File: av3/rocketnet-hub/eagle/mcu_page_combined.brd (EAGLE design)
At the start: 112.7 x 76.3 mm, 393 parts, among them J1 ROCKETNET-CONNECTOR-16M, J10 ROCKETNET-UMBILICAL-12, J11 1.27MM_HDR_2X5, J12 1.27MM_HDR_2X12X1, J2 ROCKETNET-CONNECTOR-16M, J3 ROCKETNET-CONNECTOR-16M, J4 ROCKETNET-CONNECTOR-16M, J5 1.27MM_HDR_2X12X1, J6 ROCKETNET-CONNECTOR-16M, J7 ROCKETNET-CONNECTOR-16M, J8 ROCKETNET-CONNECTOR-16M, J9 ROCKETNET-BATTERY-14, Q1 25MHz, Q2 FDS6680ASOIC-8, Q3 FDS6680ASOIC-8, Q4 FDS6680ASOIC-8, Q5 SIS412DNSOP-8, Q6 BSS138W-7-F, Q7 SIS412DNSOP-8, U1 STM32F407V100-PIN_QFP, U2 BQ24725QFN-20

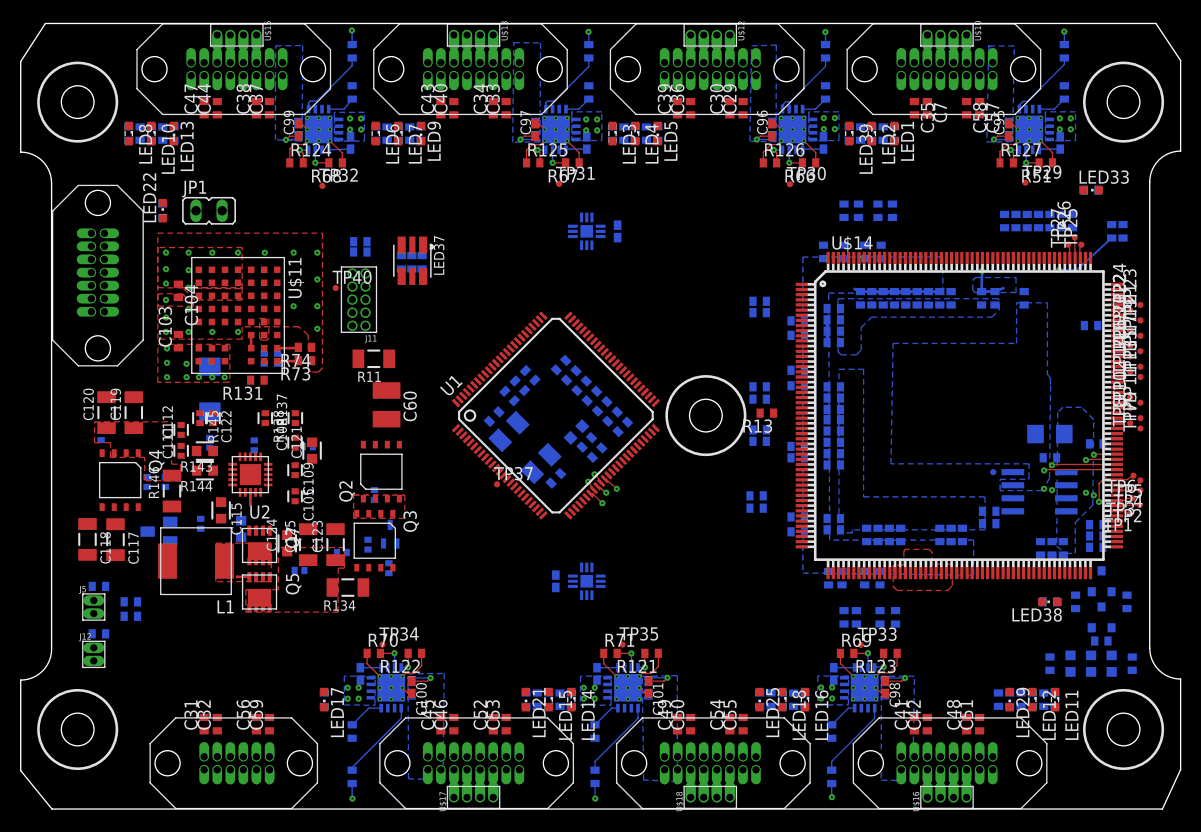
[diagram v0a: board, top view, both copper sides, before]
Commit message: Fixed ground vias DRC errors
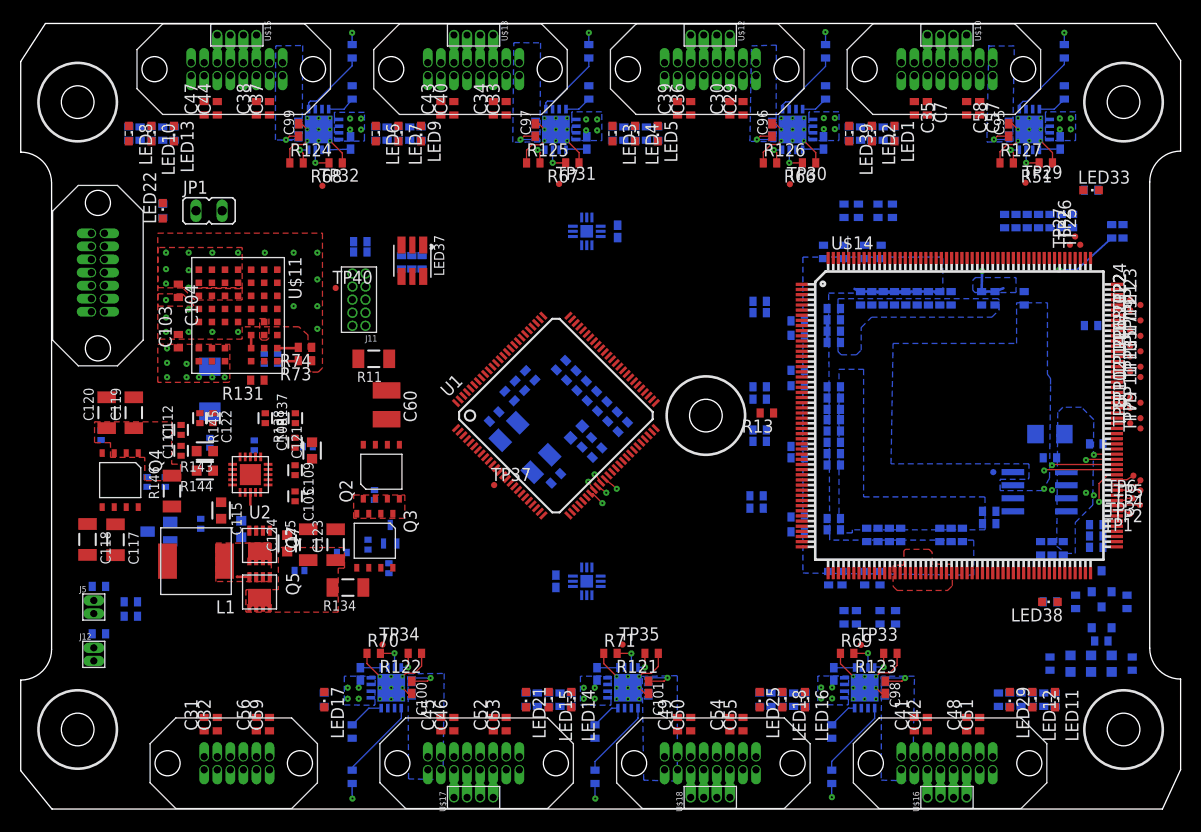
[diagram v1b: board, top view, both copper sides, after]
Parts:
- moved TP37 0.30 mm to (46.0, 31.4)
- moved TP27 0.19 mm to (102.0, 54.7)
- moved TP25 0.11 mm to (103.0, 54.7)
- moved TP26 0.10 mm to (102.5, 55.5)
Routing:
- net N$95: track 2.01 -> 0.00 mm
- net N$93: track 1.38 -> 0.00 mm
- net N$97: track 1.37 -> 0.00 mm
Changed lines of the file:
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@@
 <layers>
 <layer number="1" name="Top" color="4" fill="1" visible="yes" active="yes"/>
-<layer number="2" name="GND" color="1" fill="3" visible="no" active="yes"/>
+<layer number="2" name="GND" color="1" fill="3" visible="yes" active="yes"/>
 <layer number="3" name="Power" color="4" fill="3" visible="no" active="yes"/>
 <layer number="14" name="NS" color="1" fill="6" visible="yes" active="yes"/>
@@
 <attribute name="TP_SIGNAL_NAME" value="" x="107.8" y="49.35" size="1.778" layer="27" rot="R90" display="off"/>
 </element>
-<element name="TP25" library="testpad" package="TP06R" value="TPTP06R" x="103.063" y="54.7096" rot="R90">
-<attribute name="TP_SIGNAL_NAME" value="" x="103.063" y="54.7096" size="1.778" layer="27" rot="R90" display="off"/>
+<element name="TP25" library="testpad" package="TP06R" value="TPTP06R" x="102.95" y="54.7" rot="R90">
+<attribute name="TP_SIGNAL_NAME" value="" x="102.95" y="54.7" size="1.778" layer="27" rot="R90" display="off"/>
 </element>
-<element name="TP26" library="testpad" package="TP06R" value="TPTP06R" x="102.413" y="55.4096" rot="R90">
-<attribute name="TP_SIGNAL_NAME" value="" x="102.413" y="55.4096" size="1.778" layer="27" rot="R90" display="off"/>
+<element name="TP26" library="testpad" package="TP06R" value="TPTP06R" x="102.45" y="55.5" rot="R90">
+<attribute name="TP_SIGNAL_NAME" value="" x="102.45" y="55.5" size="1.778" layer="27" rot="R90" display="off"/>
 </element>
-<element name="TP27" library="testpad" package="TP06R" value="TPTP06R" x="101.763" y="54.7096" rot="R90">
-<attribute name="TP_SIGNAL_NAME" value="" x="101.763" y="54.7096" size="1.778" layer="27" rot="R90" display="off"/>
+<element name="TP27" library="testpad" package="TP06R" value="TPTP06R" x="101.95" y="54.7" rot="R90">
+<attribute name="TP_SIGNAL_NAME" value="" x="101.95" y="54.7" size="1.778" layer="27" rot="R90" display="off"/>
 </element>
 <element name="R2" library="rcl" package="R0402" value="10" x="106" y="56" rot="MR90"/>
@@
 </element>
 <element name="D3" library="diode-0603" package="0603-B-NOSILK-DIODE" value="DIODE-0603" x="104" y="14" rot="MR90"/>
-<element name="TP37" library="testpad" package="TP06R" value="TPTP06R" x="46.2876" y="31.4218">
-<attribute name="TP_SIGNAL_NAME" value="" x="46.0876" y="31.4218" size="1.778" layer="27" display="off"/>
+<element name="TP37" library="testpad" package="TP06R" value="TPTP06R" x="46" y="31.35">
+<attribute name="TP_SIGNAL_NAME" value="" x="45.8" y="31.35" size="1.778" layer="27" display="off"/>
 </element>
 <element name="JP1" library="jumper" package="JP1" value="" x="18.3" y="58" rot="R270"/>
@@
 <wire x1="52.04038125" y1="42.540378125" x2="53.923328125" y2="47.094396875" width="0" layer="19" extent="1-16"/>
 </signal>
-<signal name="GND" class="1" airwireshidden="yes">
+<signal name="GND" class="1">
 <contactref element="U1" pad="10"/>
 <contactref element="C1" pad="2"/>
@@
 <wire x1="27" y1="66.45" x2="27.295" y2="66.448" width="0.127" layer="1"/>
 <wire x1="27.295" y1="66.448" x2="27.85" y2="65.9" width="0.127" layer="1"/>
-<wire x1="32.2" y1="74.15" x2="32.2" y2="75.5142" width="0.127" layer="16"/>
-<wire x1="32.2" y1="75.5142" x2="32.1818" y2="75.5142" width="0.127" layer="16"/>
-<via x="32.1818" y="75.5142" extent="1-16" drill="0.2032" diameter="0.6096"/>
 <wire x1="32.1818" y1="75.5142" x2="32.1818" y2="75.7174" width="0.127" layer="2"/>
-<wire x1="32.1818" y1="75.7174" x2="32.2072" y2="75.7174" width="0.127" layer="2"/>
-<wire x1="55.2" y1="74.15" x2="55.2" y2="75.3872" width="0.127" layer="16"/>
-<wire x1="55.2" y1="75.3872" x2="55.1688" y2="75.3872" width="0.127" layer="16"/>
-<via x="55.1688" y="75.3872" extent="1-16" drill="0.2032" diameter="0.6096"/>
-<wire x1="55.1688" y1="75.3872" x2="55.1688" y2="75.4634" width="0.127" layer="2"/>
+<wire x1="32.1818" y1="75.7174" x2="32.2" y2="75.7174" width="0.127" layer="2"/>
 <wire x1="78.2" y1="74.15" x2="78.2" y2="75.343" width="0.127" layer="16"/>
 <wire x1="78.2" y1="75.343" x2="78.1812" y2="75.3618" width="0.127" layer="16"/>
@@
 <wire x1="78.1812" y1="75.3618" x2="78.1812" y2="75.438" width="0.127" layer="2"/>
 <wire x1="78.1812" y1="75.438" x2="78.2066" y2="75.4634" width="0.127" layer="2"/>
-<wire x1="101.4" y1="74.15" x2="101.4" y2="75.4126" width="0.127" layer="16"/>
-<wire x1="101.4" y1="75.4126" x2="101.3968" y2="75.4126" width="0.127" layer="16"/>
-<via x="101.3968" y="75.4126" extent="1-16" drill="0.2032" diameter="0.6096"/>
-<wire x1="101.3968" y1="75.4126" x2="101.3968" y2="75.5142" width="0.127" layer="2"/>
 <wire x1="32.2" y1="2.35" x2="32.2" y2="0.889" width="0.127" layer="16"/>
 <wire x1="32.2" y1="0.889" x2="32.2326" y2="0.889" width="0.127" layer="16"/>
@@
 <vertex x="81.9" y="30.2"/>
 </polygon>
-<wire x1="99.1" y1="64.8" x2="99.04" y2="63.99" width="0" layer="19" extent="16-16"/>
+<wire x1="32.2" y1="74.15" x2="32.2" y2="75.3" width="0.127" layer="16"/>
+<via x="32.2" y="75.3" extent="1-16" drill="0.2032" diameter="0.6096"/>
+<wire x1="32.2" y1="75.3" x2="32.2" y2="75.7174" width="0.127" layer="2"/>
+<wire x1="32.2" y1="75.7174" x2="32.2072" y2="75.7174" width="0.127" layer="2"/>
 <wire x1="79" y1="13.6" x2="79.65" y2="14" width="0" layer="19" extent="1-16"/>
 <wire x1="56" y1="13.6" x2="56.65" y2="14" width="0" layer="19" extent="1-16"/>
 <wire x1="33" y1="13.6" x2="33.65" y2="14" width="0" layer="19" extent="1-16"/>
+<wire x1="99.04" y1="63.99" x2="99.1" y2="64.8" width="0" layer="19" extent="16-16"/>
 <wire x1="76.04" y1="63.99" x2="76.1" y2="64.8" width="0" layer="19" extent="16-16"/>
 <wire x1="53.04" y1="63.99" x2="53.1" y2="64.8" width="0" layer="19" extent="16-16"/>
@@
 <wire x1="8.25" y1="21.5" x2="12.282" y2="32.1336" width="0" layer="19" extent="16-16"/>
 <wire x1="8.25" y1="16.9" x2="8.25" y2="21.5" width="0" layer="19" extent="16-16"/>
+<wire x1="55.2" y1="74.15" x2="55.2" y2="75.3" width="0.127" layer="16"/>
+<via x="55.2" y="75.3" extent="1-16" drill="0.2032" diameter="0.6096"/>
+<wire x1="55.2" y1="75.3" x2="55.2" y2="75.4" width="0.127" layer="2"/>
+<wire x1="55.2" y1="75.4" x2="62.555" y2="72.395" width="0" layer="19" extent="1-16"/>
+<wire x1="101.4" y1="74.15" x2="101.4" y2="75.3" width="0.127" layer="16"/>
+<via x="101.4" y="75.3" extent="1-16" drill="0.2032" diameter="0.6096"/>
+<wire x1="101.4" y1="75.3" x2="101.4" y2="75.4" width="0.127" layer="2"/>
+<wire x1="101.4" y1="75.4" x2="99.1" y2="67" width="0" layer="19" extent="1-16"/>
 </signal>
 <signal name="+3V3" class="1">
@@
 <contactref element="U$14" pad="159"/>
 <contactref element="TP25" pad="TP"/>
-<wire x1="102.95" y1="53.4" x2="102.903" y2="54.5496" width="0.127" layer="1"/>
-<wire x1="102.903" y1="54.5496" x2="103.063" y2="54.7096" width="0.127" layer="1"/>
+<wire x1="102.95" y1="54.7" x2="102.95" y2="53.4" width="0" layer="19" extent="1-1"/>
 </signal>
 <signal name="N$95">
 <contactref element="U$14" pad="160"/>
 <contactref element="TP26" pad="TP"/>
-<wire x1="102.45" y1="53.4" x2="102.413" y2="55.4096" width="0.127" layer="1"/>
+<wire x1="102.45" y1="55.5" x2="102.45" y2="53.4" width="0" layer="19" extent="1-1"/>
 </signal>
 <signal name="N$97">
 <contactref element="U$14" pad="161"/>
 <contactref element="TP27" pad="TP"/>
-<wire x1="101.763" y1="54.7096" x2="101.903" y2="54.5696" width="0.127" layer="1"/>
-<wire x1="101.903" y1="54.5696" x2="101.95" y2="53.4" width="0.127" layer="1"/>
+<wire x1="101.95" y1="54.7" x2="101.95" y2="53.4" width="0" layer="19" extent="1-1"/>
 </signal>
 <signal name="N$100">
@@
 <contactref element="R148" pad="1"/>
 <wire x1="46.8946875" y1="32.28758125" x2="102" y2="14.8" width="0" layer="19" extent="1-16"/>
-<wire x1="46.2876" y1="31.4218" x2="46.8946875" y2="32.28758125" width="0" layer="19" extent="1-1"/>
+<wire x1="46" y1="31.35" x2="46.8946875" y2="32.28758125" width="0" layer="19" extent="1-1"/>
 <wire x1="32.23" y1="51.905" x2="46.8946875" y2="32.28758125" width="0" layer="19" extent="1-1"/>
 <wire x1="32.35" y1="54" x2="32.23" y2="51.905" width="0" layer="19" extent="16-16"/>
-<wire x1="20.365" y1="4.955" x2="46.2876" y2="31.4218" width="0" layer="19" extent="1-1"/>
+<wire x1="20.365" y1="4.955" x2="46" y2="31.35" width="0" layer="19" extent="1-1"/>
 <wire x1="20.365" y1="3.685" x2="20.365" y2="4.955" width="0" layer="19" extent="1-1"/>
 <wire x1="11.35" y1="18.6" x2="20.365" y2="4.955" width="0" layer="19" extent="16-16"/>
